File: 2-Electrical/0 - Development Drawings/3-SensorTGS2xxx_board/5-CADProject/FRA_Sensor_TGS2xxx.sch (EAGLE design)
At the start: 68 parts, among them IC1 LMV611, IC3 LMV796MF_NOPB, IC4 LMP91000SD_NOPB, IC5 REF3125AQDBZRQ1, IC6 MCP6541T-I_OT, J1 INSERT_MM5_06691.5MM, J10 2wire, J2 TGS3, J3 TGS2, J4 TGS1, J5 TGS4, J6 INSERT_MM5_06691.5MM, J7 INSERT_MM5_06691.5MM, J8 INSERT_MM5_06691.5MM, J9 INSERT_MM5_06691.5MM, Q1 PMBFJ177,215, Q3 Si2300DS, X1 3-ELECTRODE-GAS-SENSORINS

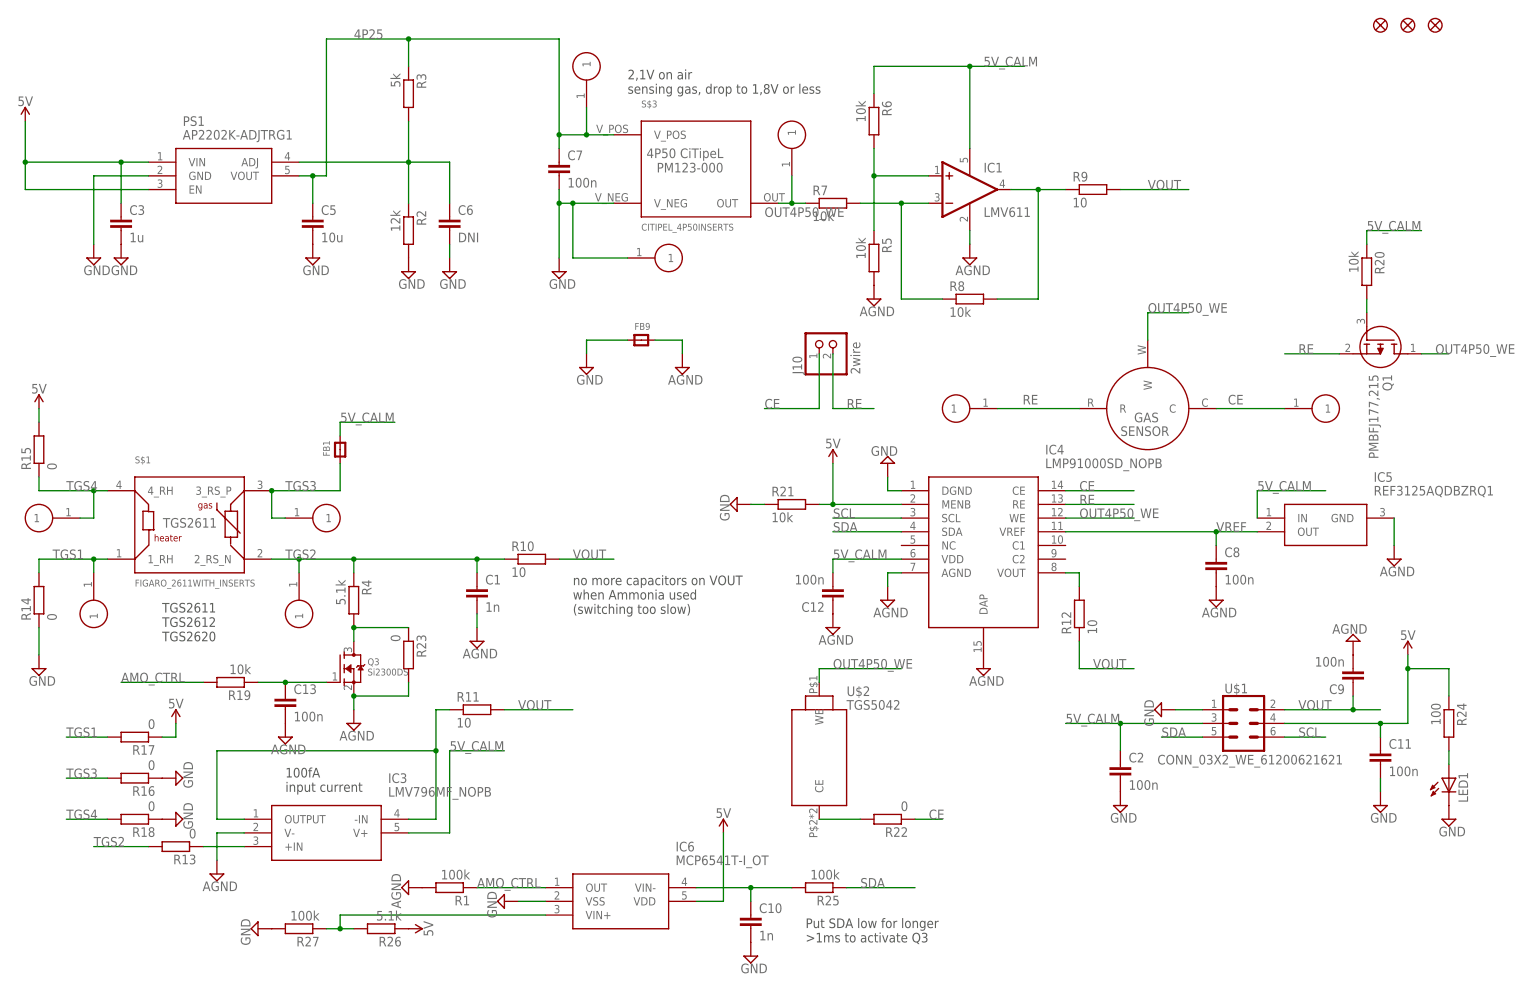
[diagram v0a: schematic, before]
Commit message: hw design updates
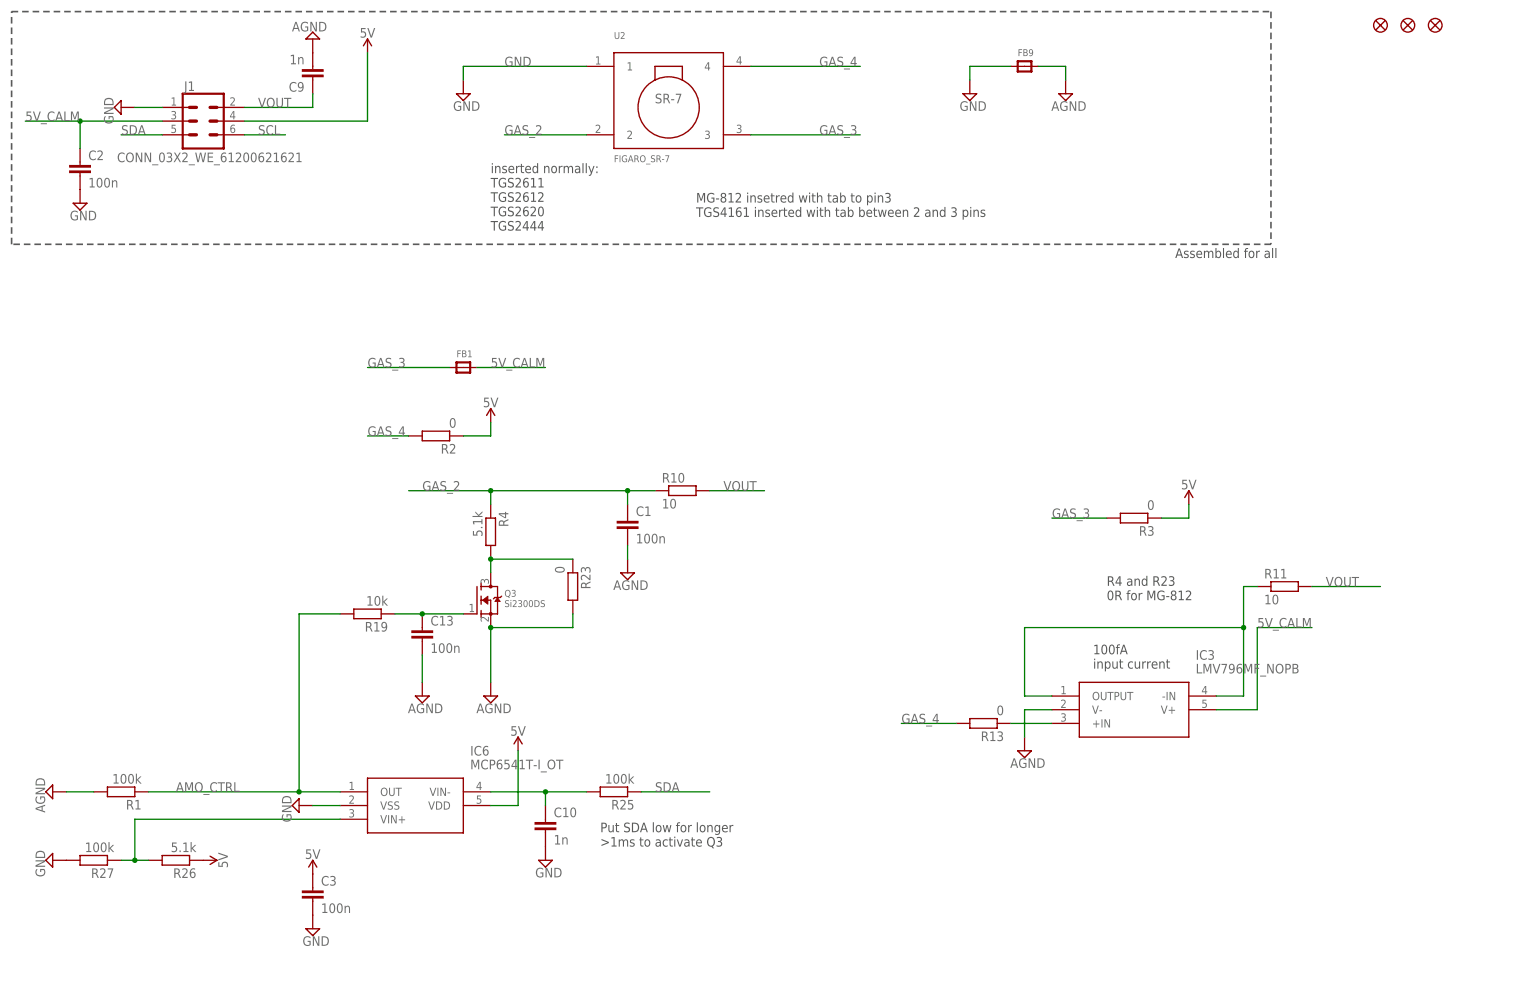
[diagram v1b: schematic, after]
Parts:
- removed C11, C12, C7, C8: 100n, resistor:C-EUC0603K
- removed C5: 10u, resistor:C-EUC0603K
- removed C6: DNI, resistor:C-EUC0603K
- removed IC1: LMV611, linear:OPA333DCK
- removed IC4: LMP91000SD_NOPB, SamacSys_Parts:LMP91000SD_NOPB
- removed IC5: REF3125AQDBZRQ1, SamacSys_Parts:REF3125AQDBZRQ1
- removed J10: 2wire, pinhead:PINHD-1X2
- removed J2: TGS3, FRA_eagle_lib:INSERT_MM5_0669
- removed J3: TGS2, FRA_eagle_lib:INSERT_MM5_0669
- removed J4: TGS1, FRA_eagle_lib:INSERT_MM5_0669
- removed J5: TGS4, FRA_eagle_lib:INSERT_MM5_0669
- removed J6, J7, J8, J9: INSERT_MM5_06691.5MM, FRA_eagle_lib:INSERT_MM5_06691.5MM
- removed LED1: (no value), adafruit:LEDCHIP-LED0603
- removed PS1: AP2202K-ADJTRG1, SamacSys_Parts:AP2202K-ADJTRG1
- removed Q1: PMBFJ177,215, SamacSys_Parts:PMBFJ177,215
- removed R12, R9: 10, resistor:R-EU_R0603
- removed R14, R15, R16, R17, R18, R22: 0, resistor:R-EU_R0603
- removed R20, R21, R5, R6, R7, R8: 10k, resistor:R-EU_R0603
- removed R24: 100, resistor:R-EU_R0603
- removed S$1: FIGARO_2611WITH_INSERTS, FRA_eagle_lib:FIGARO_2611WITH_INSERTS
- removed S$3: CITIPEL_4P50INSERTS, FRA_eagle_lib:CITIPEL_4P50INSERTS
- removed U$1: CONN_03X2_WE_61200621621, FRA_eagle_lib:CONN_03X2_WE_61200621621
- removed U$2: TGS5042, FRA_eagle_lib:TGS5042
- removed X1: 3-ELECTRODE-GAS-SENSORINS, gas-sensor:3-ELECTRODE-GAS-SENSORINS
- added U2: FIGARO_SR-7, FRA_eagle_lib:FIGARO_SR-7
- C1: value 1n -> 100n
- C3: value 1u -> 100n
- C9: value 100n -> 1n
- J1: value INSERT_MM5_06691.5MM -> CONN_03X2_WE_61200621621; device FRA_eagle_lib:INSERT_MM5_06691.5MM -> FRA_eagle_lib:CONN_03X2_WE_61200621621
- R2: value 12k -> 0
- R3: value 5k -> 0
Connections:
- removed net 4P25: C5.1, C7.1, J6.1, PS1.VOUT, R3.1, S$3.V_POS
- removed net CE: IC4.CE, J10.1, J9.1, R22.1, X1.C
- removed net N$1: LED1.A, R24.2
- removed net N$19: R22.2, U$2.CE
- removed net N$2: C6.1, PS1.ADJ, R2.1, R3.2
- removed net N$3: IC4.VOUT, R12.2
- removed net N$4: IC1.+IN, R5.1, R6.2
- removed net N$5: IC1.-IN, R7.2, R8.1
- removed net N$6: IC1.OUT, R8.2, R9.1
- removed net N$9: Q1.G, R20.2
- removed net OUT4P50_WE: IC4.WE, J7.1, Q1.D, R7.1, S$3.OUT, U$2.WE, X1.W
- removed net RE: IC4.RE, J10.2, J8.1, Q1.S, X1.R
- removed net TGS1: J4.1, R14.2, R17.2, S$1.1_RH
- removed net TGS2: C1.1, J3.1, R10.1, R13.2, R4.1, S$1.2_RS_N
- removed net TGS3: FB1.P$1, J2.1, R16.2, S$1.3_RS_P
- removed net TGS4: J5.1, R15.1, R18.2, S$1.4_RH
- removed net VREF: C8.1, IC4.VREF, IC5.OUT
- new net GAS_2: C1.1, R10.1, R4.1, U2.2
- new net GAS_3: FB1.P$1, R3.2, U2.3
- new net GAS_4: R13.2, R2.2, U2.4
- net 5V: now also J1.4, R2.1, R3.1; no longer C11.1, IC4.MENB, PS1.EN, PS1.VIN, R15.2, R17.1, R21.2, R24.1, U$1.4
- net 5V_CALM: now also J1.3; no longer C12.2, IC1.V+, IC4.VDD, IC5.IN, R20.1, R6.1, U$1.3
- net AGND: no longer C12.1, C8.2, IC1.V-, IC4.AGND, IC4.DAP, IC5.GND, R5.2
- net GND: now also U2.1; no longer C11.2, C5.2, C6.2, C7.2, IC4.DGND, LED1.C, PS1.GND, R14.1, R16.1, R18.1, R2.2, R21.1, S$3.V_NEG, U$1.1
- net SCL: now also J1.6; no longer IC4.SCL, U$1.6
- net SDA: now also J1.5; no longer IC4.SDA, U$1.5
- net VOUT: now also J1.2; no longer R12.1, R9.2, U$1.2
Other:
- note added: "Assembled for all"
- note added: "MG-812 insetred with tab to pin3 TGS4161 inserted with tab between 2 and 3 pins"
- note added: "R4 and R23 0R for MG-812"
- note added: "inserted normally: TGS2611 TGS2612 TGS2620 TGS2444"
- note removed: "2,1V on air sensing gas, drop to 1,8V or less"
- note removed: "TGS2611 TGS2612 TGS2620"
- note removed: "no more capacitors on VOUT when Ammonia used (switching too slow)"
- moved on the sheet: C1, C10, C13, C2, C3, C9, FB1, FB9, IC3, IC6, Q3, R1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
